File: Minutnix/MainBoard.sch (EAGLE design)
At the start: 121 parts, among them IC3 TP4056, IC7 FT232RL, Q4 32.768kHz, X1 FH12-12S-0.5S_THINNER, X2 JST-XH-03-PIN-LONG-PAD, X4 JST-XH-03-PIN-LONG-PAD

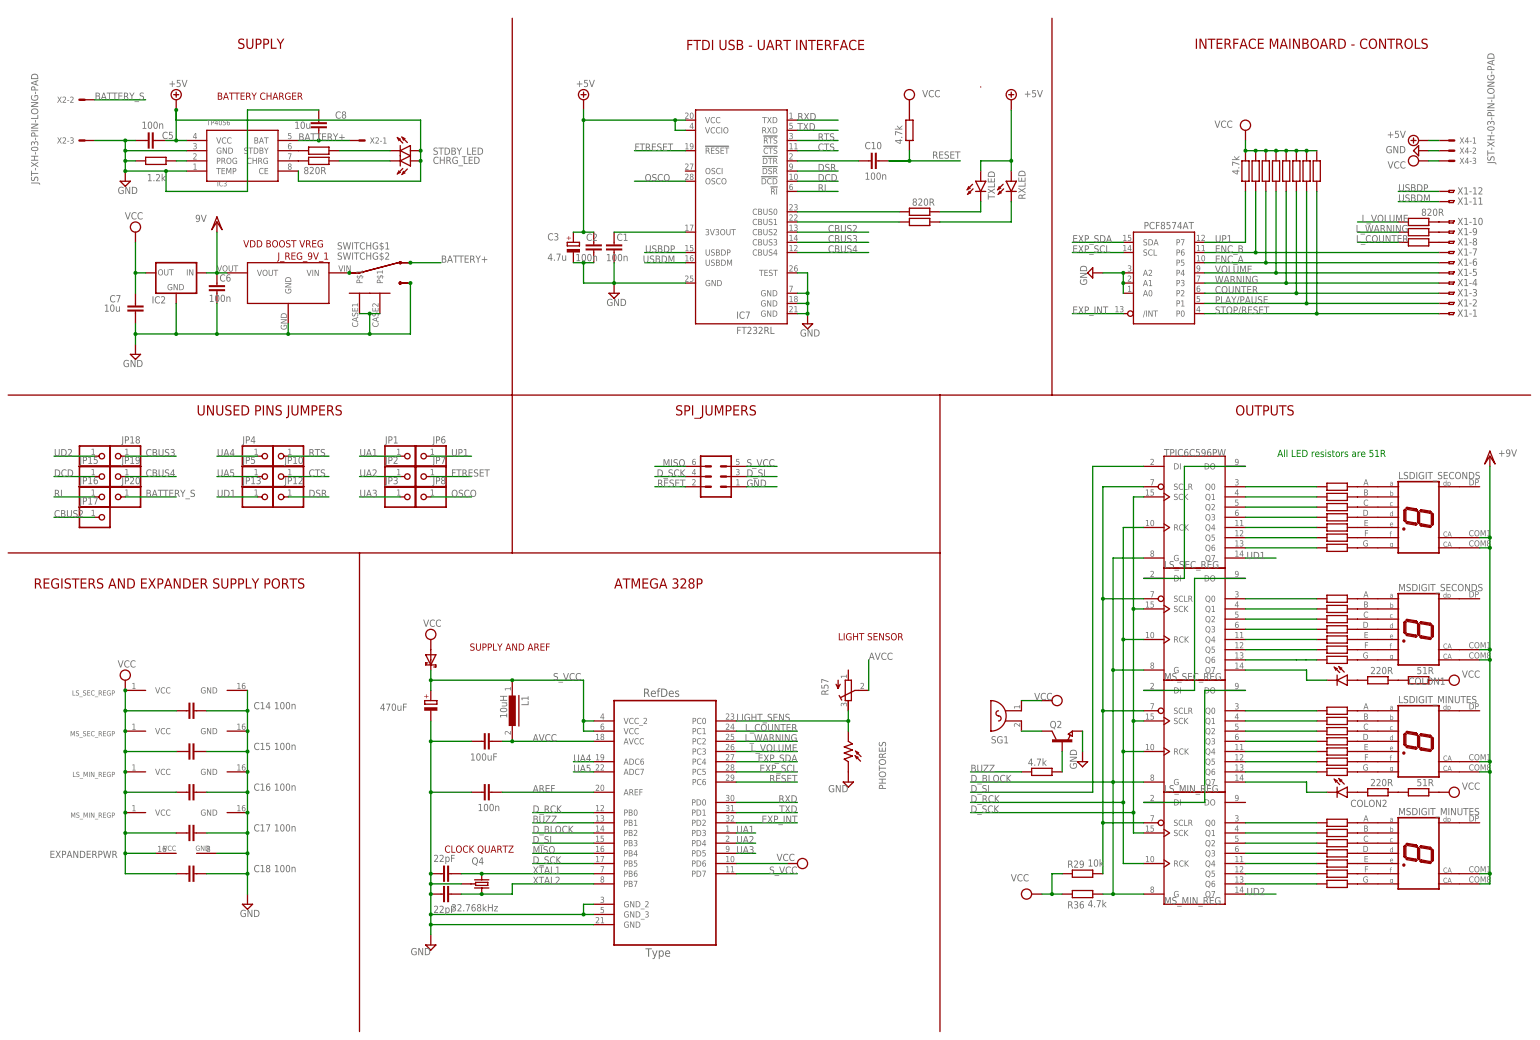
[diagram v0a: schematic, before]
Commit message: Mixing led signals
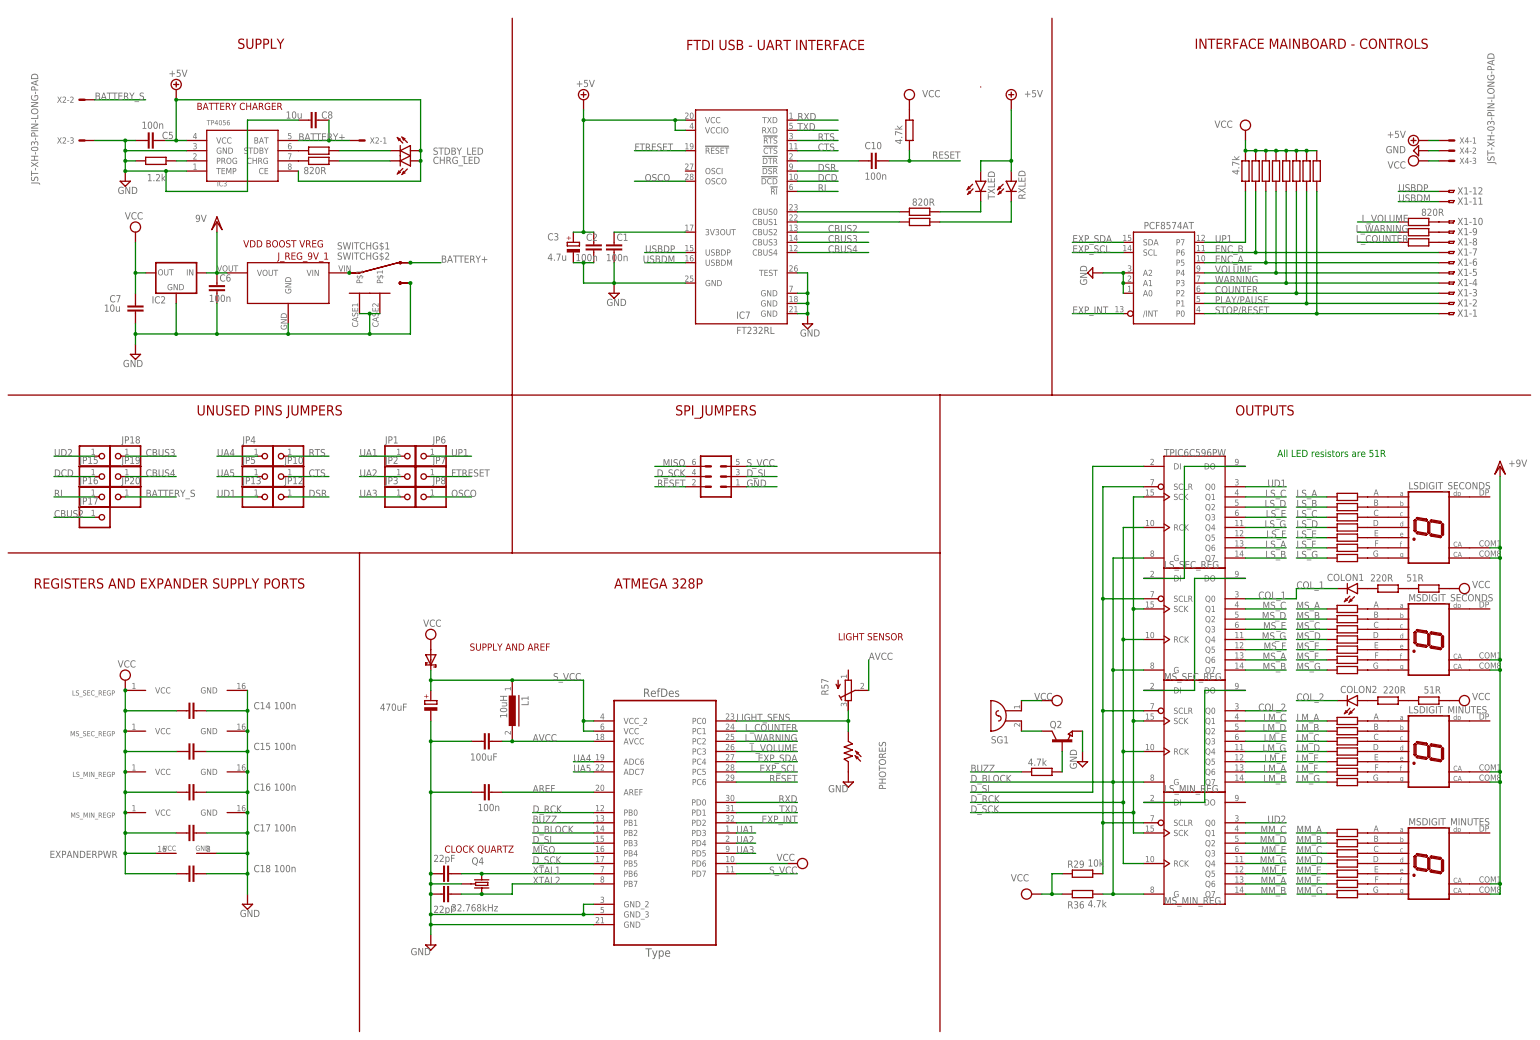
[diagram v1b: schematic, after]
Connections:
- net N$10 renamed LS_F
- net N$62 renamed MS_F
- net N$72 renamed LM_F
- net N$95 renamed MM_F
- removed net N$11: LS_SEC_REGG$1.Q6, R15.2
- removed net N$2: COLON1.C, MS_SEC_REGG$1.Q7
- removed net N$20: COLON2.C, LS_MIN_REGG$1.Q7
- removed net N$22: MS_MIN_REGG$1.Q0, R27.2
- removed net N$4: MS_SEC_REGG$1.Q0, R14.2
- removed net N$5: LS_SEC_REGG$1.Q0, R21.2
- removed net N$58: MS_SEC_REGG$1.Q1, R13.2
- removed net N$59: MS_SEC_REGG$1.Q2, R12.2
- removed net N$6: LS_SEC_REGG$1.Q1, R20.2
- removed net N$60: MS_SEC_REGG$1.Q3, R11.2
- removed net N$61: MS_SEC_REGG$1.Q4, R10.2
- removed net N$63: MS_SEC_REGG$1.Q6, R8.2
- removed net N$67: LS_MIN_REGG$1.Q0, R7.2
- removed net N$68: LS_MIN_REGG$1.Q1, R6.2
- removed net N$69: LS_MIN_REGG$1.Q2, R5.2
- removed net N$7: LS_SEC_REGG$1.Q2, R19.2
- removed net N$70: LS_MIN_REGG$1.Q3, R4.2
- removed net N$71: LS_MIN_REGG$1.Q4, R3.2
- removed net N$73: LS_MIN_REGG$1.Q6, R1.2
- removed net N$75: MS_MIN_REGG$1.Q1, R26.2
- removed net N$76: MS_MIN_REGG$1.Q2, R25.2
- removed net N$77: MS_MIN_REGG$1.Q3, R24.2
- removed net N$8: LS_SEC_REGG$1.Q3, R18.2
- removed net N$9: LS_SEC_REGG$1.Q4, R17.2
- removed net N$94: MS_MIN_REGG$1.Q4, R23.2
- removed net N$96: MS_MIN_REGG$1.Q6, R28.2
- new net COL_1: COLON1.C, MS_SEC_REGG$1.Q0
- new net COL_2: COLON2.C, LS_MIN_REGG$1.Q0
- new net LM_A: LS_MIN_REGG$1.Q6, R7.2
- new net LM_B: LS_MIN_REGG$1.Q7, R6.2
- new net LM_C: LS_MIN_REGG$1.Q1, R5.2
- new net LM_D: LS_MIN_REGG$1.Q2, R4.2
- new net LM_E: LS_MIN_REGG$1.Q3, R3.2
- new net LM_G: LS_MIN_REGG$1.Q4, R1.2
- new net LS_A: LS_SEC_REGG$1.Q6, R21.2
- new net LS_B: LS_SEC_REGG$1.Q7, R20.2
- new net LS_C: LS_SEC_REGG$1.Q1, R19.2
- new net LS_D: LS_SEC_REGG$1.Q2, R18.2
- new net LS_E: LS_SEC_REGG$1.Q3, R17.2
- new net LS_G: LS_SEC_REGG$1.Q4, R15.2
- new net MM_A: MS_MIN_REGG$1.Q6, R27.2
- new net MM_B: MS_MIN_REGG$1.Q7, R26.2
- new net MM_C: MS_MIN_REGG$1.Q1, R25.2
- new net MM_D: MS_MIN_REGG$1.Q2, R24.2
- new net MM_E: MS_MIN_REGG$1.Q3, R23.2
- new net MM_G: MS_MIN_REGG$1.Q4, R28.2
- new net MS_A: MS_SEC_REGG$1.Q6, R14.2
- new net MS_B: MS_SEC_REGG$1.Q7, R13.2
- new net MS_C: MS_SEC_REGG$1.Q1, R12.2
- new net MS_D: MS_SEC_REGG$1.Q2, R11.2
- new net MS_E: MS_SEC_REGG$1.Q3, R10.2
- new net MS_G: MS_SEC_REGG$1.Q4, R8.2
- net UD1: now also LS_SEC_REGG$1.Q0; no longer LS_SEC_REGG$1.Q7
- net UD2: now also MS_MIN_REGG$1.Q0; no longer MS_MIN_REGG$1.Q7
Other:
- moved on the sheet: C8, COLON1, COLON2, LSDIGIT_MINUTES, LSDIGIT_SECONDS, MSDIGIT_MINUTES, MSDIGIT_SECONDS
